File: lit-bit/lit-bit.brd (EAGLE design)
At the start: 37.5 x 49.5 mm, 71 parts, among them J2 USB_MICRO_B_SMD_FEMALE, J3 ISP, U2 32U4, U3 73831, U4 ADXL345, U5 S-1335, U6 MCP7940N, U7 24FC1025, Y1 8MHz, Y2 32.768kHz, Y3 32.768kHz, Y4 16MHz

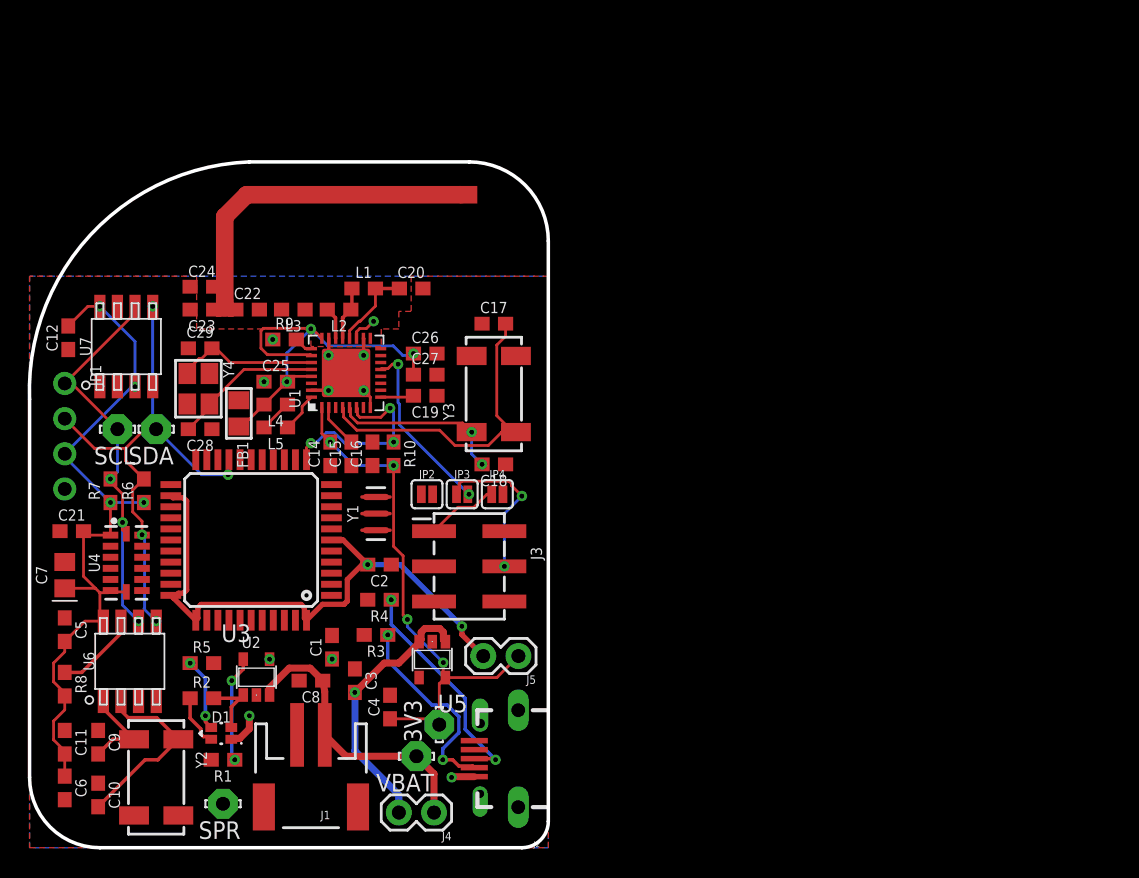
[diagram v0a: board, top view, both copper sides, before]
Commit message: reworking
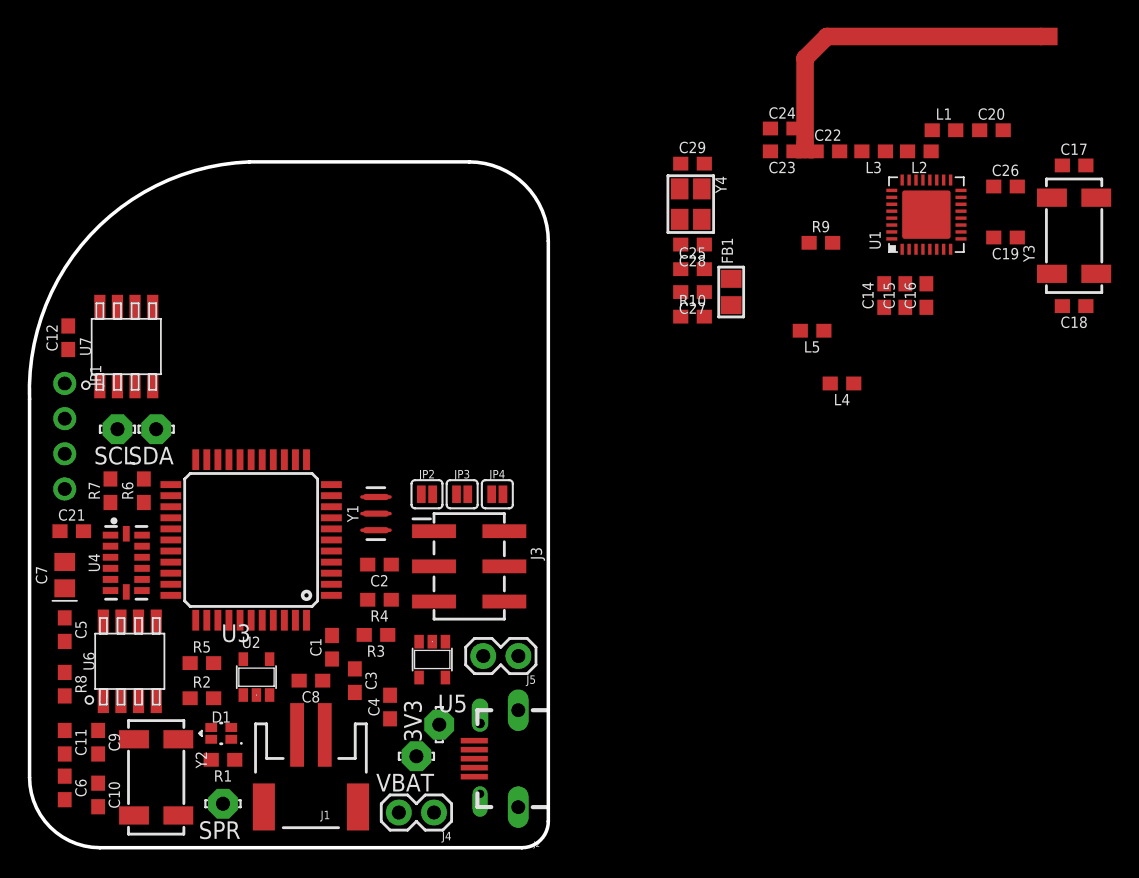
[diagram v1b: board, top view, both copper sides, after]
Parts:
- moved C26 43.6 mm to (69.8, 47.8)
- moved C17 43.4 mm to (74.8, 49.3)
- moved C20 43.4 mm to (68.8, 51.8)
- moved C22 43.4 mm to (57.0, 50.3)
- moved L2 43.4 mm to (63.6, 50.3)
- moved L3 43.4 mm to (60.3, 50.3)
- moved U1 43.4 mm to (64.1, 45.7)
- moved C18 43.4 mm to (74.8, 39.1)
- moved C19 43.4 mm to (69.8, 44.1)
- moved C23 43.4 mm to (53.7, 50.3)
- moved C24 43.4 mm to (53.7, 51.9)
- moved L1 43.4 mm to (65.4, 51.8)
- moved U$28 43.4 mm to (55.4, 50.4)
- moved Y3 43.4 mm to (74.8, 44.2)
- moved C16 41.6 mm to (64.1, 39.9)
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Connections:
- net ACTIVE: no longer R10.1
- net RDYN: now also R10.1
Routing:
- net 3V3: track 94.8 -> 0.00 mm, vias 8 -> 0
- net ITSYPWR: track 43.1 -> 0.00 mm, vias 2 -> 0
- net SDA: track 39.2 -> 0.00 mm, vias 4 -> 0
- net AVDD: track 31.5 -> 0.00 mm, vias 3 -> 0
- net SCL: track 28.8 -> 0.00 mm, vias 3 -> 0
- net N$15: track 23.0 -> 0.00 mm
- net VBAT: track 21.1 -> 0.00 mm
- net VBAT-JMP: track 19.5 -> 0.00 mm, vias 1 -> 0
- net UD+: track 16.2 -> 0.00 mm, vias 2 -> 0
- net UD-: track 14.8 -> 0.00 mm, vias 2 -> 0
- net ACTIVE: track 13.8 -> 0.00 mm, vias 3 -> 0
- net N$21: track 13.5 -> 0.00 mm
- net N$29: track 13.0 -> 0.00 mm, vias 2 -> 0
- net N$23: track 12.5 -> 0.00 mm, vias 2 -> 0
- net MOSI: track 11.6 -> 0.00 mm, vias 2 -> 0
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- removed copper zone on layer 1, net GND
- removed copper zone on layer 16, net GND
